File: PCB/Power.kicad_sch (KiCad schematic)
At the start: 29 parts, among them J1 3.7v LiPo, Q1 MMBT2907ALT1HTSA1, Q2 NMOS, U1 TPS61090, U2 LD1117S33TR_SOT223, U3 MCP73831T-2ACI/OT

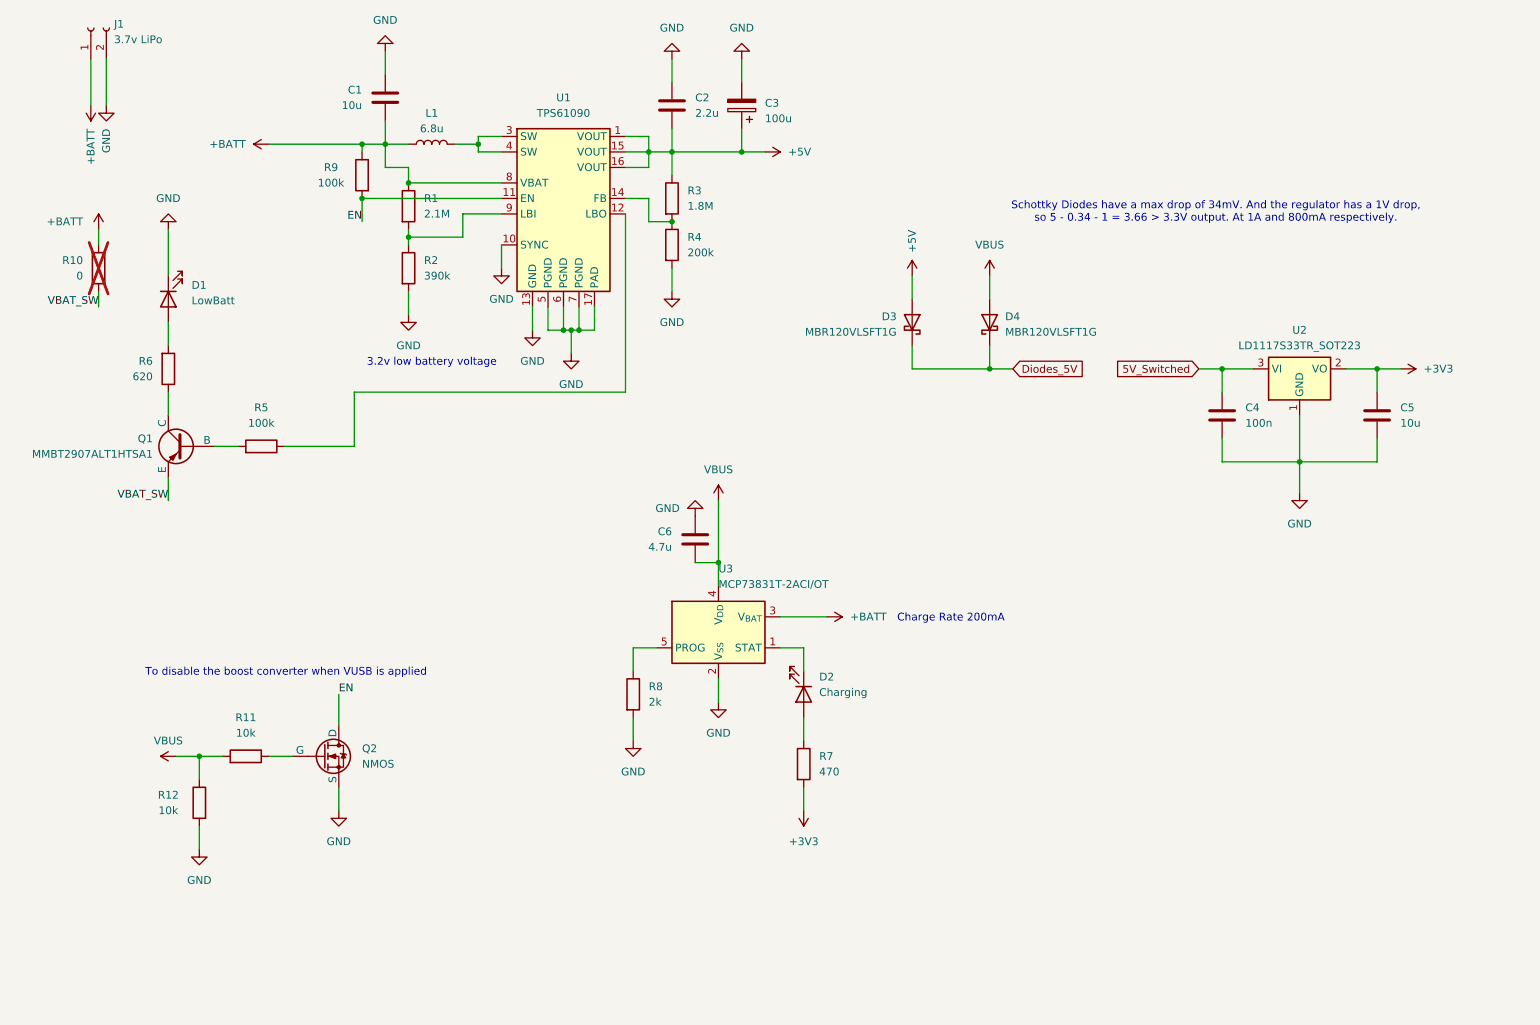
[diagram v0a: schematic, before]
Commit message: Finished the schematic.
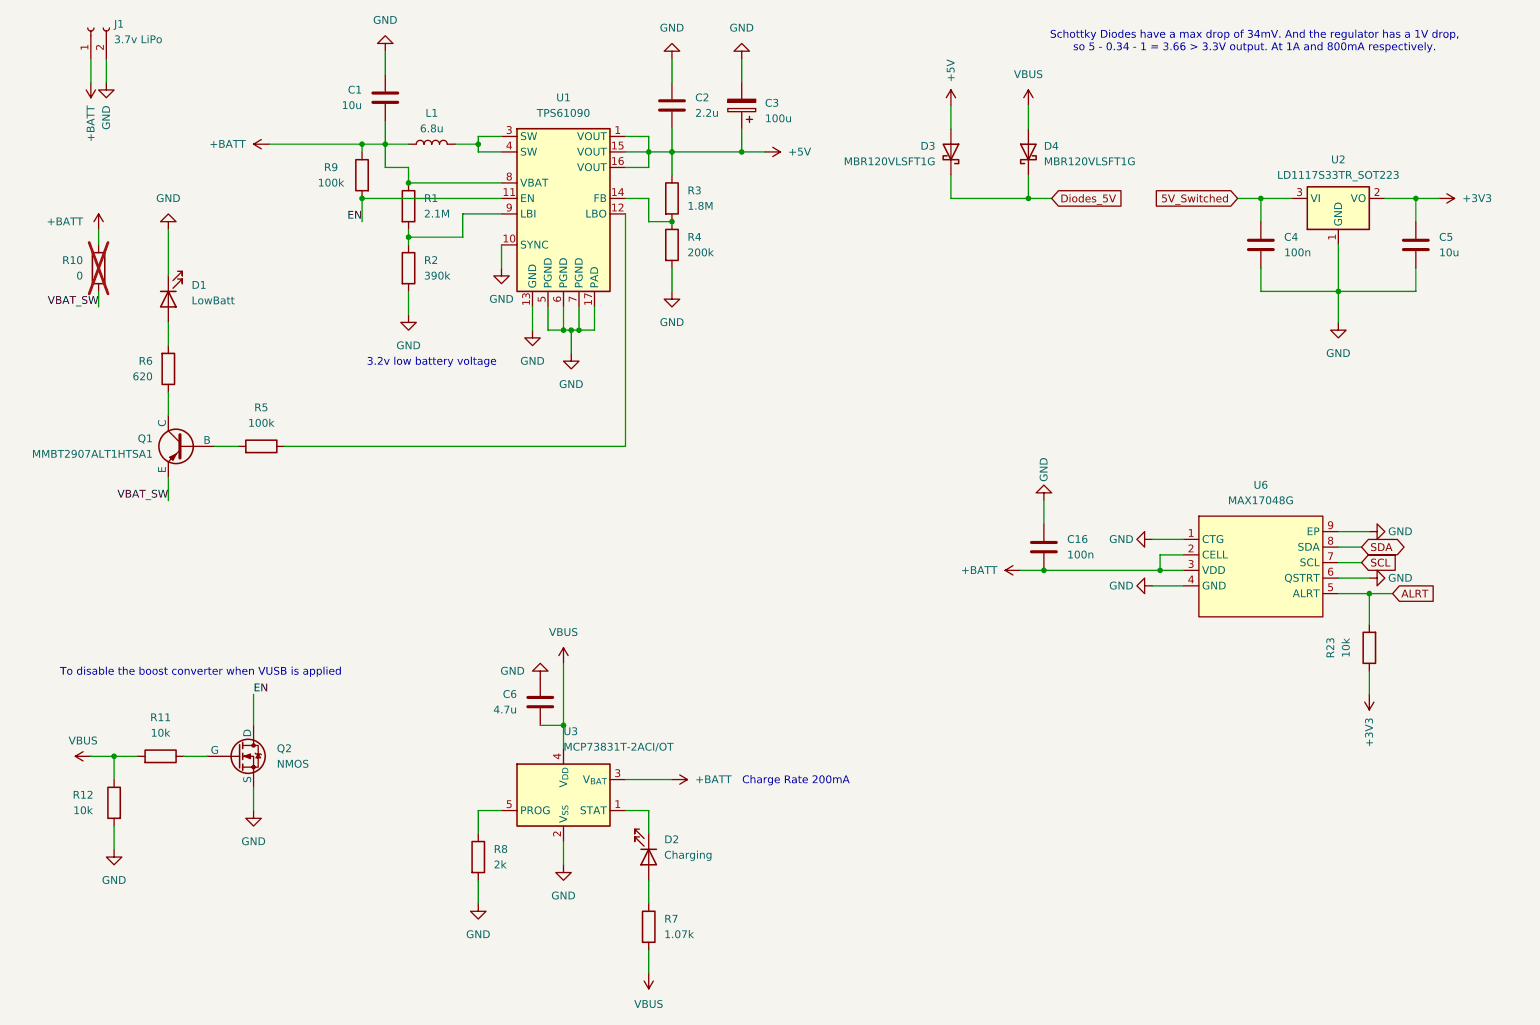
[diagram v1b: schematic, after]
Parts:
- removed C4: 100n, Capacitor_SMD:C_0201_0603Metric, symbol Device:C
- added C16: 100n, Capacitor_SMD:C_0201_0603Metric, symbol Device:C
- added R23: 10k, Resistor_SMD:R_0201_0603Metric, symbol Device:R
- added U6: MAX17048G, Package_DFN_QFN:TDFN-8-1EP_2x2mm_P0.5mm_EP0.8x1.2mm, symbol CustomSymbols:MAX17048G
- R7: value 470 -> 1.07k; LCSC C844786 -> C4217127
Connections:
- net +3V3: now also R23.1; no longer R7.2
- net +BATT: now also C16.2, U6.2 (CELL), U6.3 (VDD)
- net 5V_Switched: now also C16.1
- net GND: now also C16.1, C16.2, U6.1 (CTG), U6.4 (GND), U6.6 (QSTRT), U6.9 (EP)
- net VBUS: now also R7.2
- new net ALRT: R23.2, U6.5 (ALRT)
- new net SCL: U6.7 (SCL)
- new net SDA: U6.8 (SDA)
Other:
- moved on the sheet: C5, C6, D2, D3, D4, Q2, R11, R12, R8, U2, U3
